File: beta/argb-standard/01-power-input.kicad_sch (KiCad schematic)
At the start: 9 parts, among them J1 SATA_PWR_15P, Q1 AO4407A

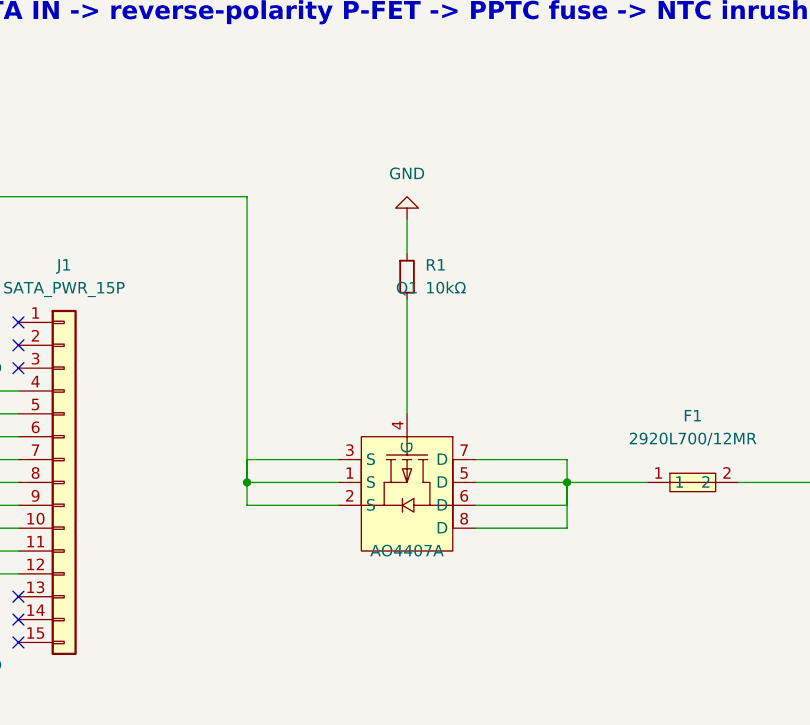
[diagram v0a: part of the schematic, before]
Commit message: Audit BETA electrical and pour pipeline
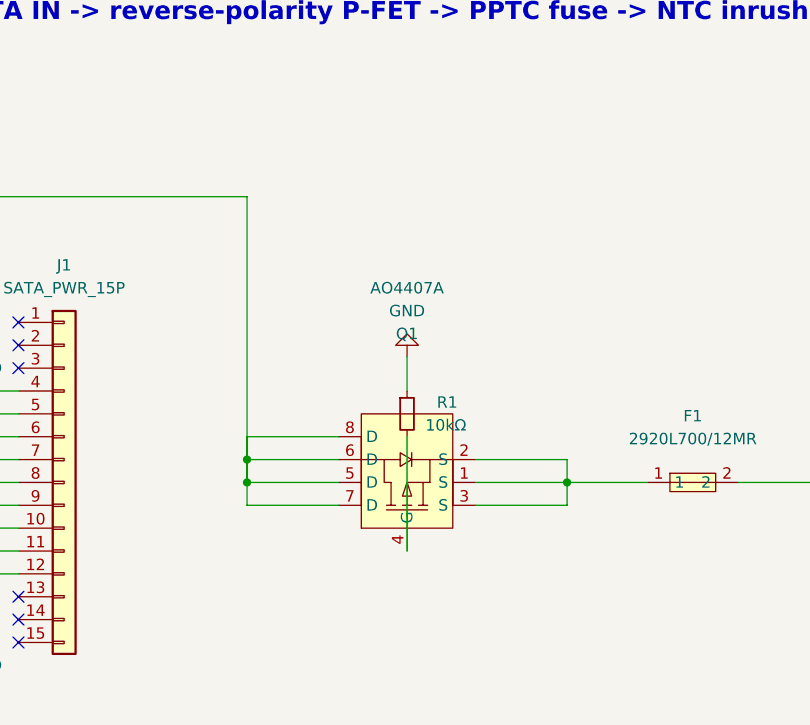
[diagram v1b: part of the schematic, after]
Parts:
- RT1: MPN MF72-5D-20 -> MF72 5D20
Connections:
- net at Q1.1 (S), Q1.2 (S), Q1.3 (S): now also F1.1; no longer J1.7 (Pin_7), J1.8 (Pin_8), J1.9 (Pin_9)
- net at Q1.5 (D), Q1.6 (D), Q1.7 (D)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: now also J1.7 (Pin_7), J1.8 (Pin_8), J1.9 (Pin_9); no longer F1.1
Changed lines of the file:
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@@
 	(symbol
 		(lib_id "cec-vendor:AO4407A")
-		(at 153.67 123.19 270)
-		(unit 1)
-		(exclude_from_sim no)
-		(in_bom yes)
-		(on_board yes)
-		(dnp no)
-		(fields_autoplaced yes)
-		(property "Reference" "Q1" (at 153.67 101.6 90) (effects (font (size 1.27 1.27))))
-		(property "Value" "AO4407A" (at 153.67 130.81 90) (effects (font (size 1.27 1.27))))
+		(at 153.67 123.19 90)
+		(unit 1)
+		(exclude_from_sim no)
+		(in_bom yes)
+		(on_board yes)
+		(dnp no)
+		(fields_autoplaced yes)
+		(property "Reference" "Q1" (at 153.67 106.68 90) (effects (font (size 1.27 1.27))))
+		(property "Value" "AO4407A" (at 153.67 101.6 90) (effects (font (size 1.27 1.27))))
 		(property "Footprint" "cec-Package_SO:SOIC-8_L4.9-W3.9-P1.27-LS6.0-BL" (at 153.67 123.19 0) (effects (font (size 1.27 1.27)) (hide yes)))
-		(property "Datasheet" "" (at 153.67 123.19 0) (effects (font (size 1.27 1.27)) (hide yes)))
+		(property "Datasheet" "https://www.aosmd.com/res/datasheets/AO4407A.pdf" (at 153.67 123.19 0) (effects (font (size 1.27 1.27)) (hide yes)))
 		(property "Manufacturer" "Alpha & Omega Semiconductor" (at 153.67 123.19 0) (effects (font (size 1.27 1.27)) (hide yes)))
 		(property "MPN" "AO4407A" (at 153.67 123.19 0) (effects (font (size 1.27 1.27)) (hide yes)))
@@
 		(property "Value" "2920L700/12MR" (at 185.42 118.36 0) (effects (font (size 1.27 1.27))))
 		(property "Footprint" "cec-Fuse_SMD:F2920" (at 185.42 123.19 0) (effects (font (size 1.27 1.27)) (hide yes)))
-		(property "Datasheet" "" (at 185.42 123.19 0) (effects (font (size 1.27 1.27)) (hide yes)))
+		(property "Datasheet" "https://www.lcsc.com/datasheet/C207092.pdf" (at 185.42 123.19 0) (effects (font (size 1.27 1.27)) (hide yes)))
 		(property "Manufacturer" "Littelfuse" (at 185.42 123.19 0) (effects (font (size 1.27 1.27)) (hide yes)))
 		(property "MPN" "2920L700/12MR" (at 185.42 123.19 0) (effects (font (size 1.27 1.27)) (hide yes)))
@@
 		(property "Value" "MF72-5D-20" (at 210.82 118.36 0) (effects (font (size 1.27 1.27))))
 		(property "Footprint" "cec-Thermistor_THT:RES-TH_L22.0-W7.0-P10.00-D1.0-S2.00" (at 210.82 123.19 0) (effects (font (size 1.27 1.27)) (hide yes)))
-		(property "Datasheet" "" (at 210.82 123.19 0) (effects (font (size 1.27 1.27)) (hide yes)))
+		(property "Datasheet" "https://www.lcsc.com/datasheet/C122780.pdf" (at 210.82 123.19 0) (effects (font (size 1.27 1.27)) (hide yes)))
 		(property "Manufacturer" "Nanjing Shiheng Electronics" (at 210.82 123.19 0) (effects (font (size 1.27 1.27)) (hide yes)))
-		(property "MPN" "MF72-5D-20" (at 210.82 123.19 0) (effects (font (size 1.27 1.27)) (hide yes)))
+		(property "MPN" "MF72 5D20" (at 210.82 123.19 0) (effects (font (size 1.27 1.27)) (hide yes)))
 		(property "LCSC" "C122780" (at 210.82 123.19 0) (effects (font (size 1.27 1.27)) (hide yes)))
 		(property "Description" "Power NTC inrush-current limiter, 5 ohm cold / 7A rated (controlled inrush element -- spec Sec 7.2; OOS at LCSC as of 2026-07-05, flagged, matches this repo's own precedent for a real-but-thin-stock part, cf. the ESP32-S3-MINI-1 pick below)" (at 210.82 123.19 0) (effects (font (size 1.27 1.27)) (hide yes)))
@@
 	(symbol
 		(lib_id "cec-vendor:R_Small")
-		(at 153.67 100.33 0)
-		(unit 1)
-		(exclude_from_sim no)
-		(in_bom yes)
-		(on_board yes)
-		(dnp no)
-		(fields_autoplaced yes)
-		(property "Reference" "R1" (at 155.702 99.06 0) (effects (font (size 1.27 1.27)) (justify left)))
-		(property "Value" "10kΩ" (at 155.702 101.6 0) (effects (font (size 1.27 1.27)) (justify left)))
-		(property "Footprint" "cec-Resistor_SMD:R_0402_1005Metric" (at 153.67 100.33 0) (effects (font (size 1.27 1.27)) (hide yes)))
-		(property "Datasheet" "" (at 153.67 100.33 0) (effects (font (size 1.27 1.27)) (hide yes)))
-		(property "Manufacturer" "UNI-ROYAL" (at 153.67 100.33 0) (effects (font (size 1.27 1.27)) (hide yes)))
-		(property "MPN" "0402WGF1002TCE" (at 153.67 100.33 0) (effects (font (size 1.27 1.27)) (hide yes)))
-		(property "LCSC" "C25744" (at 153.67 100.33 0) (effects (font (size 1.27 1.27)) (hide yes)))
+		(at 153.67 115.57 0)
+		(unit 1)
+		(exclude_from_sim no)
+		(in_bom yes)
+		(on_board yes)
+		(dnp no)
+		(fields_autoplaced yes)
+		(property "Reference" "R1" (at 156.972 114.3 0) (effects (font (size 1.27 1.27)) (justify left)))
+		(property "Value" "10kΩ" (at 155.702 116.84 0) (effects (font (size 1.27 1.27)) (justify left)))
+		(property "Footprint" "cec-Resistor_SMD:R_0402_1005Metric" (at 153.67 115.57 0) (effects (font (size 1.27 1.27)) (hide yes)))
+		(property "Datasheet" "" (at 153.67 115.57 0) (effects (font (size 1.27 1.27)) (hide yes)))
+		(property "Manufacturer" "UNI-ROYAL" (at 153.67 115.57 0) (effects (font (size 1.27 1.27)) (hide yes)))
+		(property "MPN" "0402WGF1002TCE" (at 153.67 115.57 0) (effects (font (size 1.27 1.27)) (hide yes)))
+		(property "LCSC" "C25744" (at 153.67 115.57 0) (effects (font (size 1.27 1.27)) (hide yes)))
 		(pin "1")
 		(pin "2")
@@
 	(wire (pts (xy 135.89 123.19) (xy 146.05 123.19))
 		(stroke (width 0) (type default)))
+	(wire (pts (xy 135.89 120.65) (xy 146.05 120.65))
+		(stroke (width 0) (type default)))
+	(wire (pts (xy 135.89 125.73) (xy 146.05 125.73))
+		(stroke (width 0) (type default)))
+	(wire (pts (xy 135.89 118.11) (xy 146.05 118.11))
+		(stroke (width 0) (type default)))
+	(wire (pts (xy 135.89 118.11) (xy 135.89 120.65))
+		(stroke (width 0) (type default)))
+	(wire (pts (xy 135.89 120.65) (xy 135.89 123.19))
+		(stroke (width 0) (type default)))
 	(wire (pts (xy 135.89 123.19) (xy 135.89 125.73))
 		(stroke (width 0) (type default)))
-	(wire (pts (xy 135.89 125.73) (xy 146.05 125.73))
-		(stroke (width 0) (type default)))
-	(wire (pts (xy 135.89 123.19) (xy 135.89 120.65))
-		(stroke (width 0) (type default)))
-	(wire (pts (xy 135.89 120.65) (xy 146.05 120.65))
-		(stroke (width 0) (type default)))
 	(wire (pts (xy 161.29 123.19) (xy 171.45 123.19))
 		(stroke (width 0) (type default)))
+	(wire (pts (xy 161.29 120.65) (xy 171.45 120.65))
+		(stroke (width 0) (type default)))
 	(wire (pts (xy 161.29 125.73) (xy 171.45 125.73))
 		(stroke (width 0) (type default)))
-	(wire (pts (xy 161.29 120.65) (xy 171.45 120.65))
-		(stroke (width 0) (type default)))
-	(wire (pts (xy 161.29 128.27) (xy 171.45 128.27))
-		(stroke (width 0) (type default)))
-	(wire (pts (xy 171.45 120.65) (xy 171.45 128.27))
-		(stroke (width 0) (type default)))
-	(wire (pts (xy 153.67 115.57) (xy 153.67 102.87))
-		(stroke (width 0) (type default)))
-	(wire (pts (xy 171.45 125.73) (xy 171.45 123.19))
+	(wire (pts (xy 153.67 130.81) (xy 153.67 118.11))
 		(stroke (width 0) (type default)))
 	(wire (pts (xy 171.45 123.19) (xy 180.34 123.19))
 		(stroke (width 0) (type default)))
+	(wire (pts (xy 171.45 120.65) (xy 171.45 123.19))
+		(stroke (width 0) (type default)))
+	(wire (pts (xy 171.45 123.19) (xy 171.45 125.73))
+		(stroke (width 0) (type default)))
 	(wire (pts (xy 190.5 123.19) (xy 205.74 123.19))
 		(stroke (width 0) (type default)))
@@
 	(wire (pts (xy 110.49 133.35) (xy 104.14 133.35))
 		(stroke (width 0) (type default)))
-	(wire (pts (xy 153.67 97.79) (xy 153.67 93.98))
+	(wire (pts (xy 153.67 113.03) (xy 153.67 109.22))
 		(stroke (width 0) (type default)))
 	(wire (pts (xy 226.06 151.13) (xy 226.06 154.94))
@@
 		(stroke (width 0) (type default)))
 	(junction (at 97.79 123.19) (diameter 0) (color 0 0 0 0))
+	(junction (at 135.89 120.65) (diameter 0) (color 0 0 0 0))
 	(junction (at 135.89 123.19) (diameter 0) (color 0 0 0 0))
 	(junction (at 171.45 123.19) (diameter 0) (color 0 0 0 0))
@@
 	(symbol
 		(lib_id "cec-power:GND")
-		(at 153.67 93.98 180)
-		(unit 1)
-		(exclude_from_sim no)
-		(in_bom yes)
-		(on_board yes)
-		(dnp no)
-		(property "Reference" "#PWR107" (at 153.67 91.44 0) (effects (font (size 1.27 1.27)) (hide yes)))
-		(property "Value" "GND" (at 153.67 88.9 0) (effects (font (size 1.27 1.27))))
-		(pin "1")
-		(instances
+		(at 153.67 109.22 180)
+		(unit 1)
+		(exclude_from_sim no)
+		(in_bom yes)
+		(on_board yes)
+		(dnp no)
+		(property "Reference" "#PWR107" (at 153.67 106.68 0) (effects (font (size 1.27 1.27)) (hide yes)))
+		(property "Value" "GND" (at 153.67 104.14 0) (effects (font (size 1.27 1.27))))
+		(pin "1")
+		(instances
